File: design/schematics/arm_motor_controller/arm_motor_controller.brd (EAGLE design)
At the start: 97.2 x 54.6 mm, 60 parts, among them Q1 PFET-FQP27P06, Q2 PFET-FQP27P06, Q3 NFET-FQP30N06L, Q4 NFET-FQP30N06L, Q5 PFET-FQP27P06, Q6 PFET-FQP27P06, Q7 NFET-FQP30N06L, Q8 NFET-FQP30N06L, U1 V_REG_LD1085D2

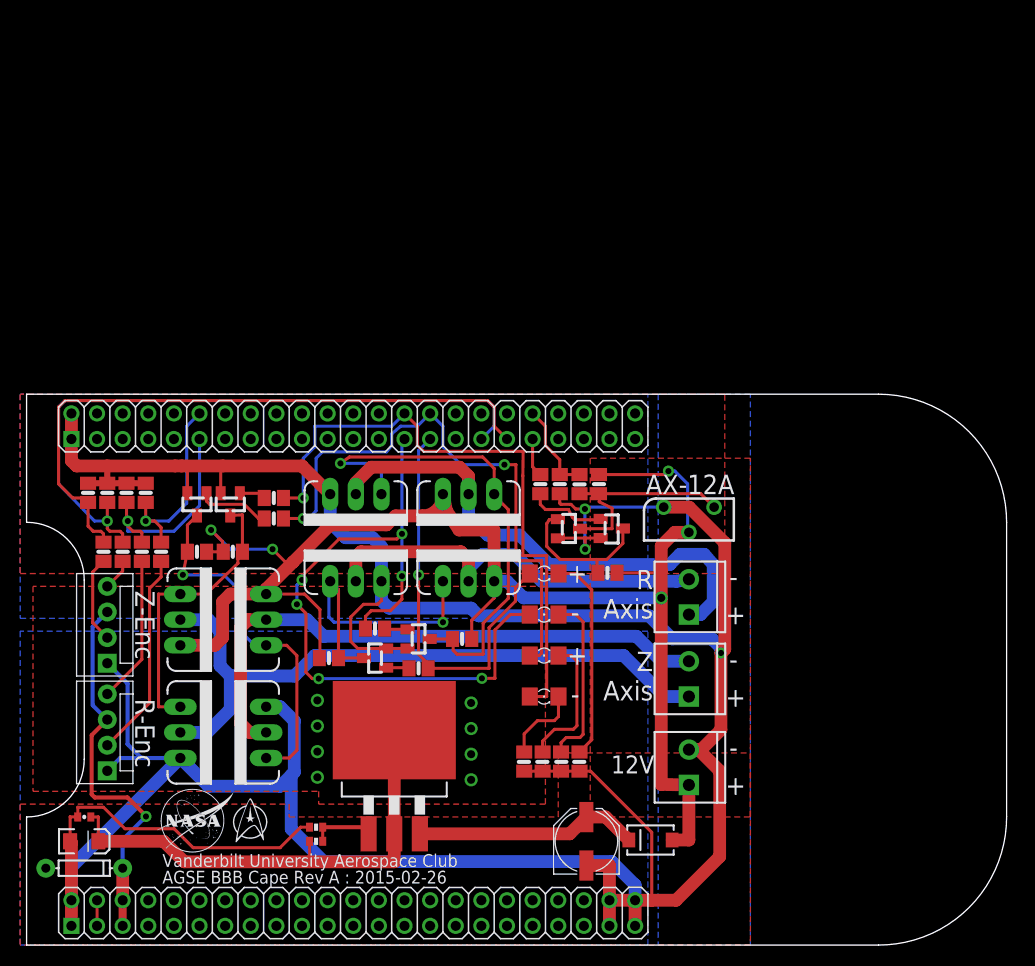
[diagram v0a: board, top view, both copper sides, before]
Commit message: working on schematic/board.
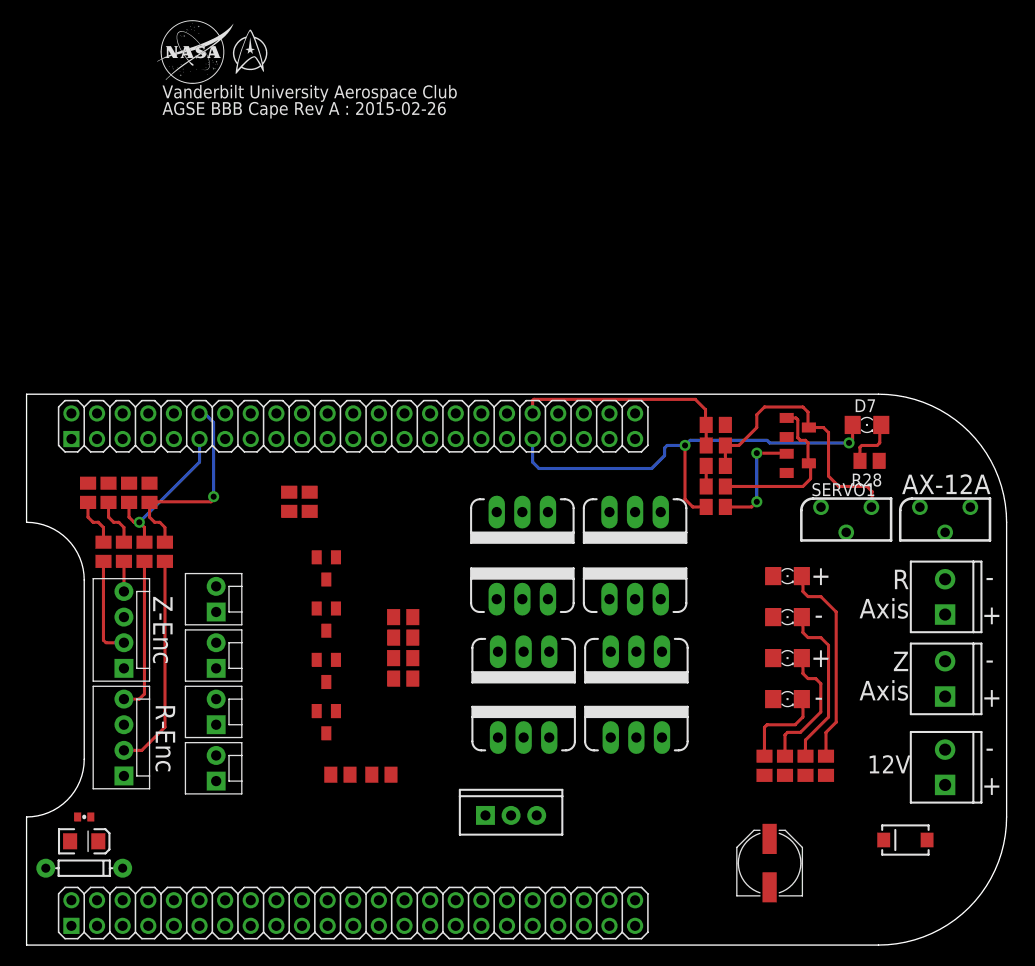
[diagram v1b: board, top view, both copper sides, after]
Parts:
- removed R1: 370, SparkFun-Passives:0402-RES
- removed R2: 1.5k, SparkFun-Passives:0402-RES
- removed U1: V_REG_LD1085D2, SparkFun-PowerIC:D2PACK/A
- added +HLS, +RLS, -HLS, -RLS: M02POLAR, SparkFun-Connectors:MOLEX-1X2
- added D7: (no value), SparkFun-LED:FKIT-LED-1206
- added LD1085: V_REG_317SINK, SparkFun-PowerIC:TO220-ADJ
- added R28: 50, resistor:M0805
- added SERVO1: AX-12A, molex-spox:SPOX-3
- moved Q7 45.2 mm to (64.5, 20.8), turned to 0 degrees
- moved Q8 37.6 mm to (64.5, 29.3), turned to 180 degrees
- moved Q5 36.0 mm to (53.3, 20.8), turned to 0 degrees
- moved Q3 29.6 mm to (64.4, 34.5), turned to 0 degrees
- moved Q4 28.5 mm to (64.4, 43.2), turned to 180 degrees
- moved R4 26.6 mm to (39.2, 17.1)
- moved R5 26.3 mm to (35.2, 17.1)
- moved Q6 25.7 mm to (53.3, 29.3), turned to 180 degrees
- moved JP1 25.4 mm to (95.1, 16.1)
- moved R-AXIS 25.4 mm to (95.1, 33.0)
- moved SERVO 25.4 mm to (95.1, 42.4)
- moved Z-AXIS 25.4 mm to (95.1, 24.9)
- moved D1 25.3 mm to (91.2, 10.7)
- moved T6 24.8 mm to (80.5, 51.6)
- moved R26 24.4 mm to (83.3, 18.0)
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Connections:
- removed net N$16: R11.2, T4.B
- removed net N$4: R1.1, R2.2, U1.1
- new net +HEIGHT_LS: +HLS.2, R7.2, T2.B, U$1.44
- new net +RADIUS_LS: +RLS.2, R11.2, T4.B, U$1.43
- new net -HEIGHT_LS: -HLS.2, R6.1, T1.B, U$1.42
- new net -RADIUS_LS: -RLS.2, R10.1, T3.B, U$1.41
- new net N$19: U$1.46
- net 12V: now also SERVO1.P$2
- net BBB_TX: now also D7.A
- net GND: now also +HLS.1, +RLS.1, -HLS.1, -RLS.1, LD1085.ADJ, R28.1, SERVO1.P$3; no longer R2.1
- net N$10: now also U$1.45; no longer R7.2, T2.B
- net N$15: now also U$1.14; no longer R10.1, T3.B
- net N$3: now also LD1085.IN; no longer U1.3
- net N$9: now also D7.C, R28.2; no longer R6.1, T1.B
- net SERVO_TX/RX: now also SERVO1.P$1
- net VOUT: now also LD1085.OUT; no longer R1.2, U1.2, U1.TAB
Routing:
- net GND: track 358.6 -> 0.00 mm, vias 3 -> 0
- net 12V: track 151.3 -> 2.03 mm, vias 4 -> 0
- net -RADIUS: track 71.2 -> 0.00 mm, vias 6 -> 0
- net Z+: track 66.6 -> 0.00 mm
- net -HEIGHT: track 61.7 -> 0.00 mm, vias 1 -> 0
- net BBB_EQEP1B: track 66.6 -> 4.87 mm, vias 1 -> 0
- net BBB_EQEP1A: track 63.9 -> 4.87 mm
- net Z-: track 58.9 -> 0.00 mm
- net +HEIGHT: track 56.9 -> 0.00 mm, vias 2 -> 0
- net R+: track 51.0 -> 0.00 mm
- net N$13: track 49.1 -> 0.00 mm, vias 1 -> 0
- net VOUT: track 48.4 -> 0.00 mm, vias 8 -> 0
- net BBB_TX: track 3.84 -> 45.3 mm, vias 0 -> 2
- net R-: track 41.1 -> 0.00 mm
- net +RADIUS: track 40.7 -> 0.00 mm, vias 1 -> 0
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- removed copper zone on layer 16, net 12V
- removed copper zone on layer 1, net GND
- removed copper zone on layer 16, net GND
- removed copper zone on layer 1, net VOUT
- removed copper zone on layer 16, net VOUT
